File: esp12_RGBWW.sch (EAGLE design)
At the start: 28 parts

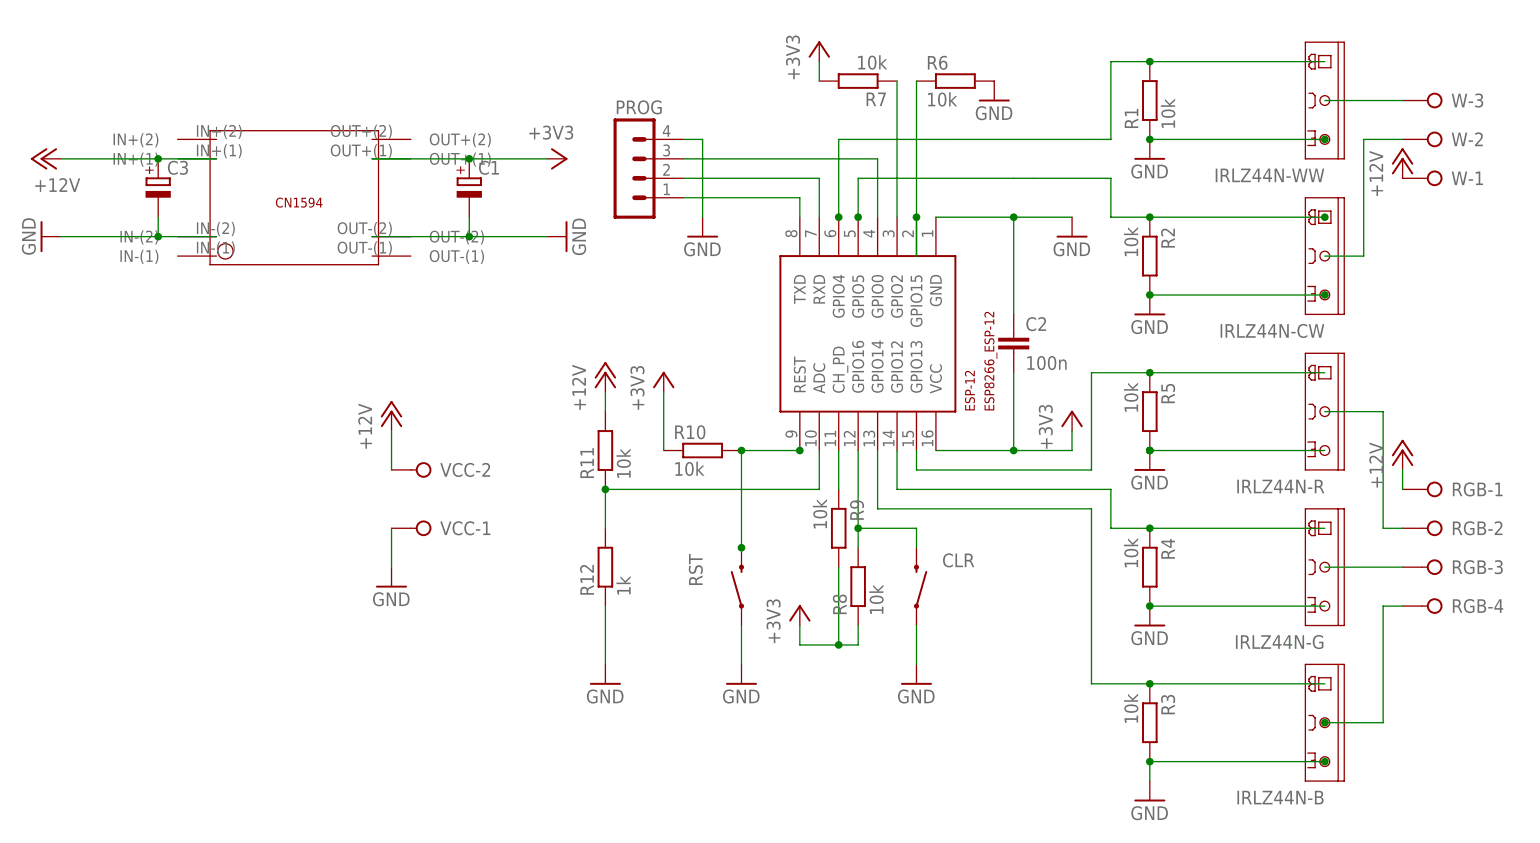
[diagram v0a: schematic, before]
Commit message: updated schematics and board v1.5
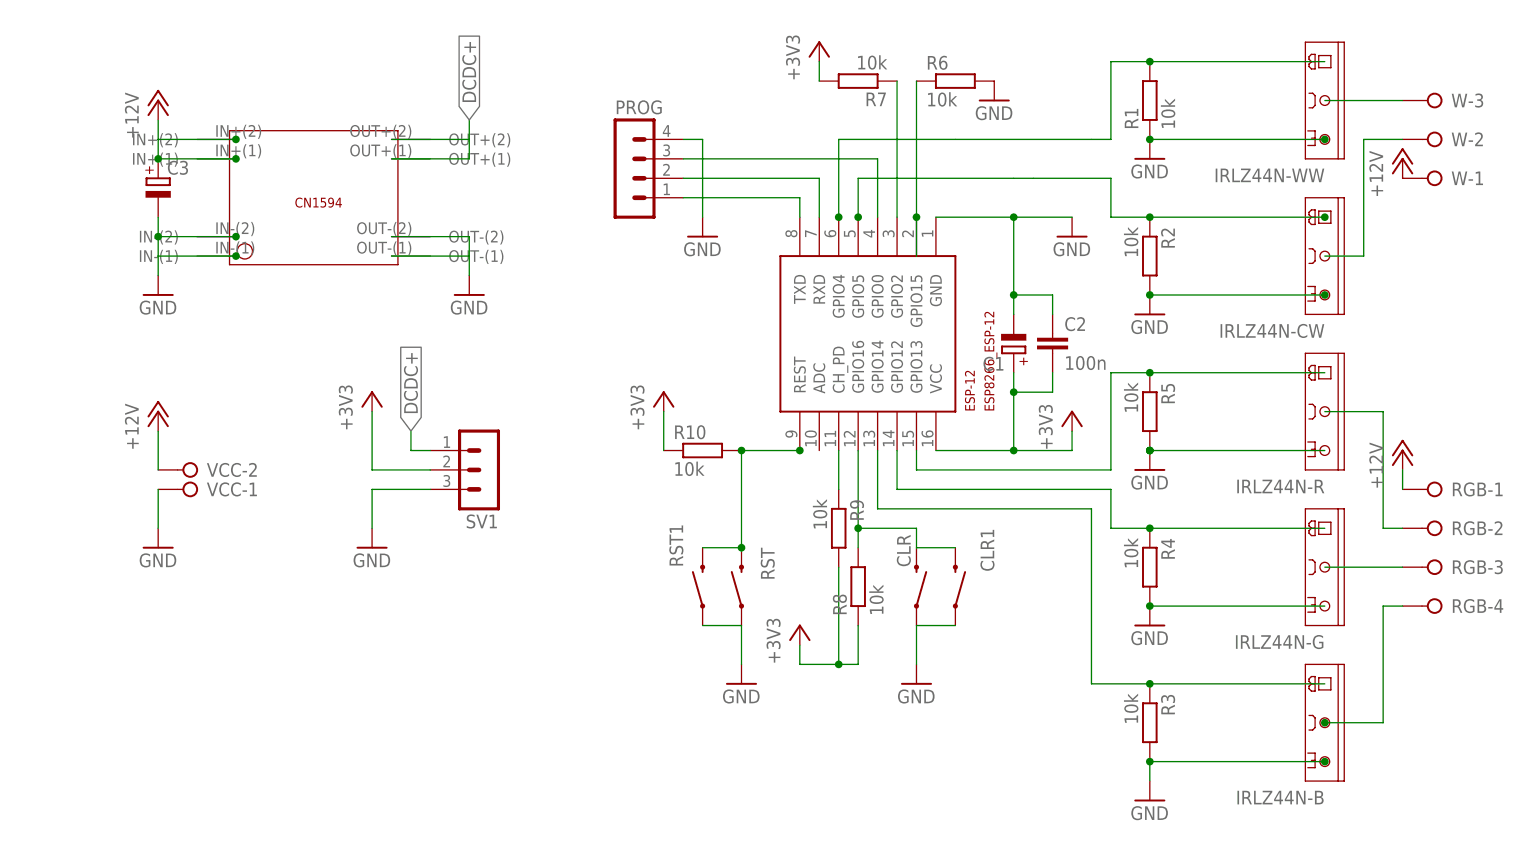
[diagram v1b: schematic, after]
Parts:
- removed DC_CONVERTER: CN1594THROUGH-HOLE, CN1594_smd:CN1594THROUGH-HOLE
- removed R11: 10k, rcl:R-EU_R0805
- removed R12: 1k, rcl:R-EU_R0805
- added CLR1, RST1: SWITCH-MOMENTARY-2SMD-1101NE, SparkFun-Electromechanical:SWITCH-MOMENTARY-2SMD-1101NE
- added SV1: (no value), con-lstb:MA03-1
- added U$2: XM1584, XM1584:XM1584
- C1: device rcl:CPOL-EUE3.5-8 -> resistor:CPOL-EUE2.5-6
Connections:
- removed net N$21: ESP-12.ADC, R11.1, R12.2
- new net DCDC+: SV1.1, U$2.OUT+(1), U$2.OUT+(2)
- net +12V: now also U$2.IN+(1), U$2.IN+(2); no longer DC_CONVERTER.IN+(1), R11.2
- net +3V3: now also SV1.2; no longer DC_CONVERTER.OUT+(1)
- net GND: now also CLR1.1, RST1.1, SV1.3, U$2.IN-(1), U$2.IN-(2), U$2.OUT-(1), U$2.OUT-(2); no longer DC_CONVERTER.IN-(2), DC_CONVERTER.OUT-(2), R12.1
- net N$1: now also CLR1.2
- net N$12: now also RST1.2
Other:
- moved on the sheet: C1, C2, VCC-1, VCC-2
